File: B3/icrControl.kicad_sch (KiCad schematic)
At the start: 11 parts, among them U329 74HC00, U330 74HC74, U331 74HC74, U332 74HC74, U333 74HC74, U334 74HC74, U335 74HC04, U336 74HC244, U337 74HC08, U338 74HC32, U339 74HC08

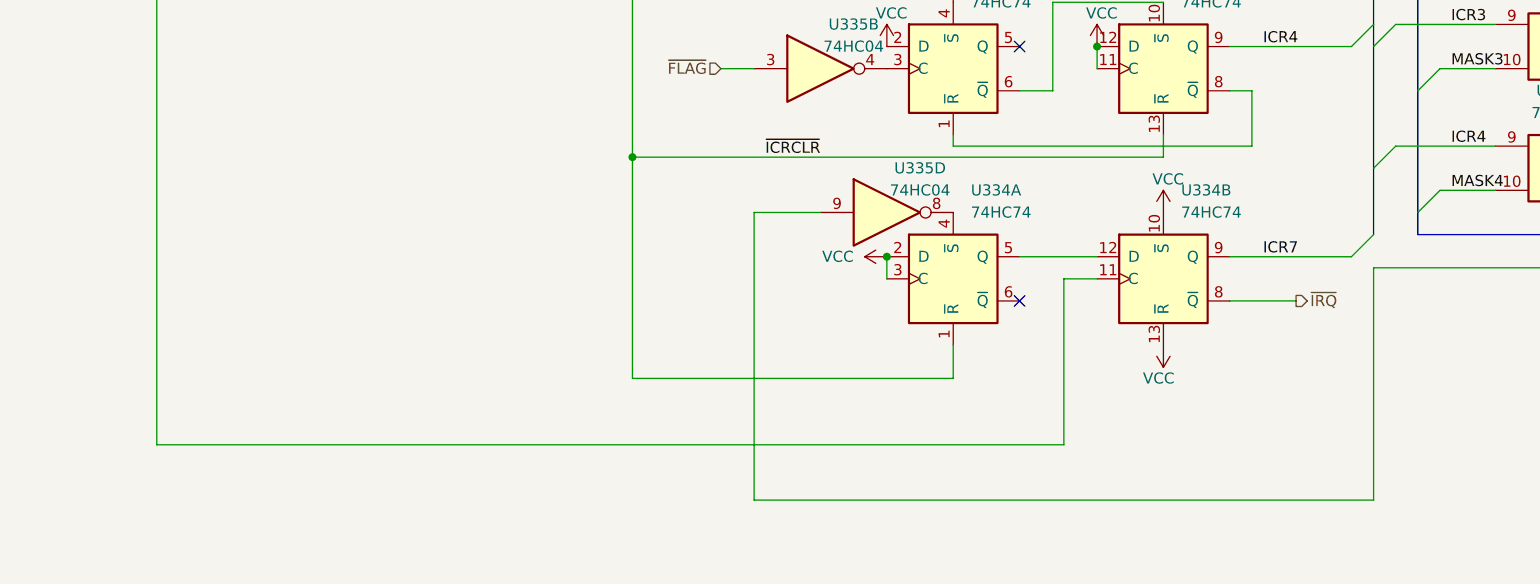
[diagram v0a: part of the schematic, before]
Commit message: Ready for v0.2.1
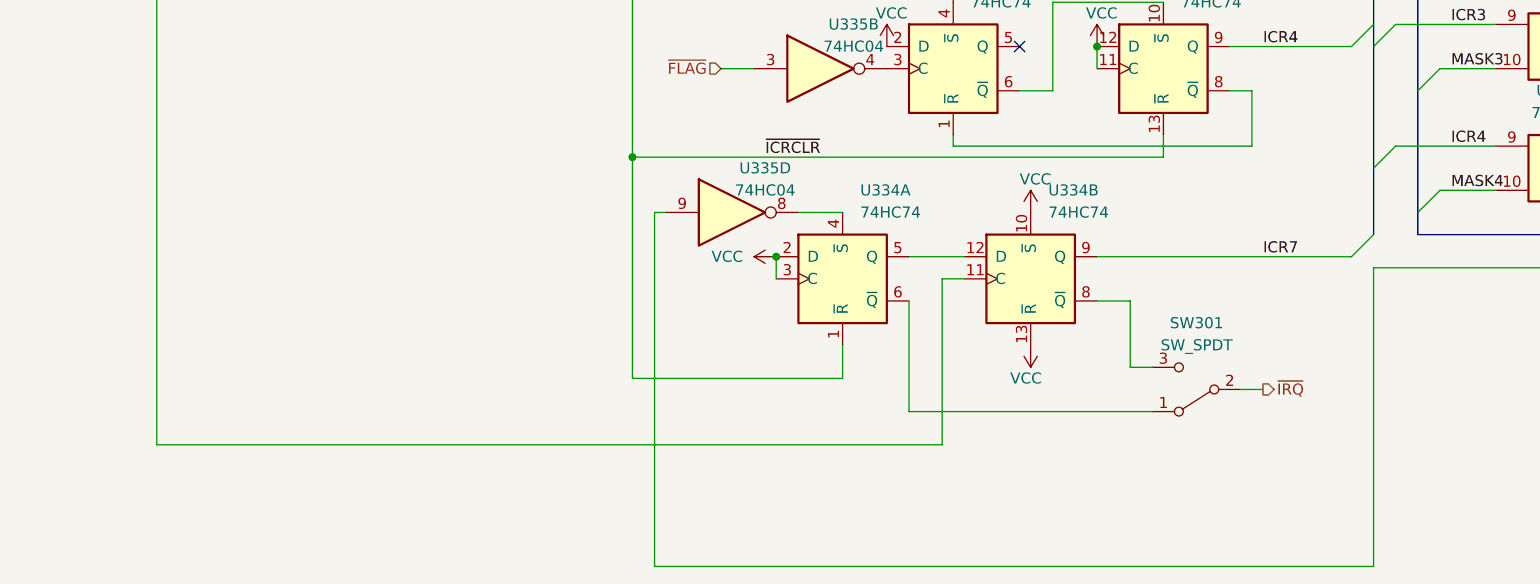
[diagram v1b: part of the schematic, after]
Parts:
- added SW301: SW_SPDT, Button_Switch_SMD:SW_SPDT_PCM12, symbol Switch:SW_SPDT
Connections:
- net ~{IRQ}: now also SW301.2 (B); no longer U334.8 (~{Q})
- net at U334.6 (~{Q}): now also SW301.1 (A)
- new net: SW301.3 (C), U334.8 (~{Q})
- no-connect marks 8 -> 7
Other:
- moved on the sheet: U334A, U334B, U335D
